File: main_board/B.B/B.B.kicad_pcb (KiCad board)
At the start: 4 copper layers, 196 x 98 mm, 249 parts, among them J2 Conn_01x10, J3 Conn_01x10, J5 USB_C_Receptacle_USB2.0, M1 Motor_DC, Q1 2N7002, Q10 2N7002, Q11 SI3447CDV, Q12 2N7002, Q2 2N7002, Q3 AO3400A, Q4 SI3447CDV, Q5 SI3447CDV, Q6 2N7002, Q7 SI3447CDV, Q8 2N7002, Q9 SI3447CDV, SW1 SW_DIP_x01, SW2 SW_DIP_x01, SW3 SW_DIP_x01, SW4 SW_DIP_x02, U1 WS2812, U10 WS2812, U11 WS2812, U12 WS2812, U13 WS2812, U14 WS2812, U15 WS2812, U16 WS2812, U17 WS2812, U18 WS2812, U19 WS2812, U2 WS2812, U20 WS2812, U21 WS2812, U22 WS2812, U23 WS2812, U24 WS2812, U25 WS2812, U26 WS2812, U27 WS2812, U28 WS2812, U29 WS2812, U3 WS2812, U30 WS2812, U31 WS2812, U32 WS2812, U33 WS2812, U34 WS2812, U35 WS2812, U36 WS2812, U37 WS2812, U38 WS2812, U39 WS2812, U4 WS2812, U40 WS2812, U41 WS2812, U42 WS2812, U43 WS2812, U44 WS2812, U45 WS2812, U46 WS2812, U47 WS2812, U48 WS2812, U49 WS2812, U5 WS2812, U50 WS2812, U51 WS2812, U52 WS2812, U53 WS2812, U54 WS2812, U55 WS2812, U56 WS2812, U57 WS2812, U58 WS2812, U59 WS2812, U6 WS2812, U60 WS2812, U61 BMX055, U62 AOZ1280, U63 FP6276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

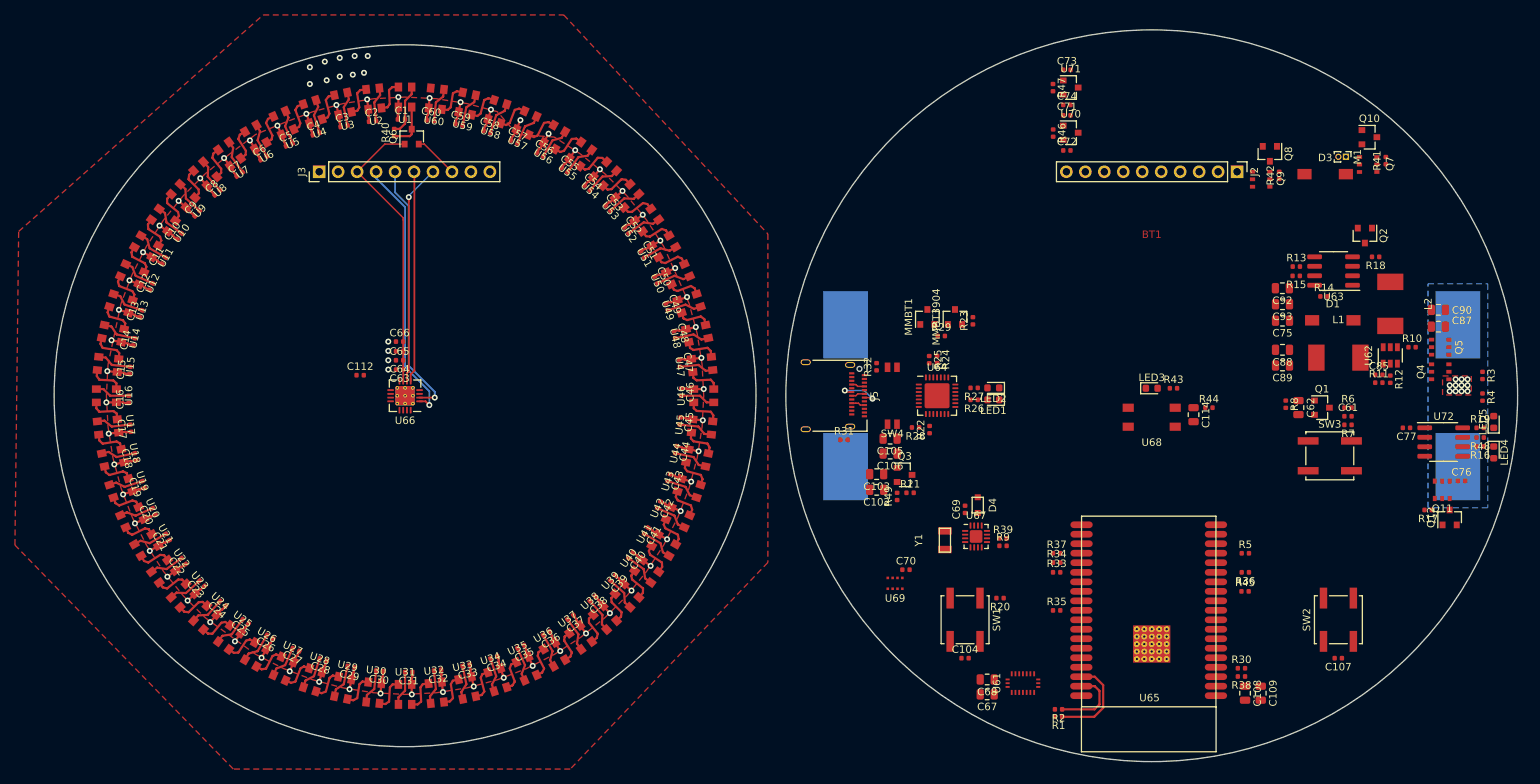
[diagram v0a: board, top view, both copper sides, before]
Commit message: PCB-0,1
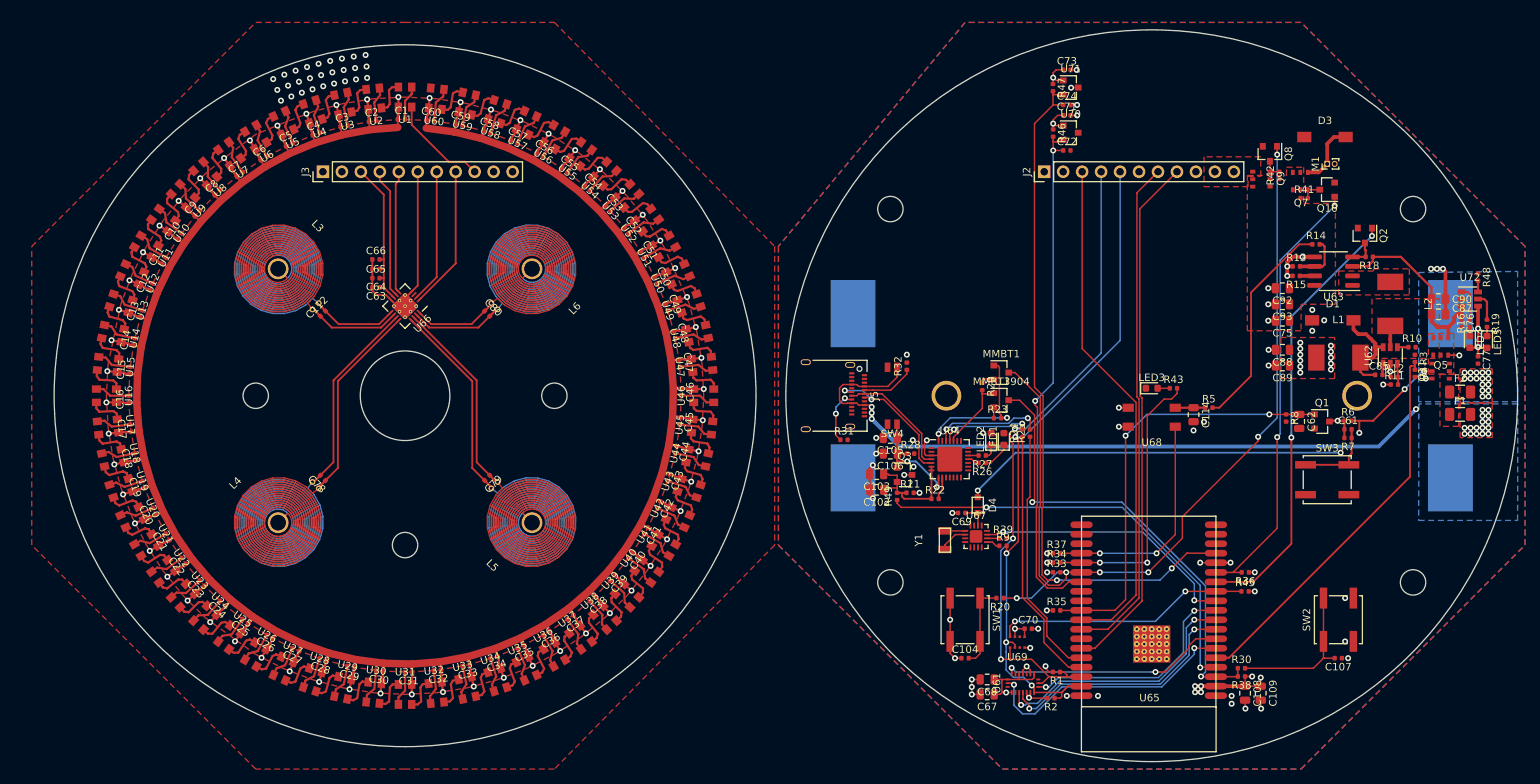
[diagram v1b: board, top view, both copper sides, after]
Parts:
- removed Q12, Q6: 2N7002, Package_TO_SOT_SMD:SOT-23
- removed Q4: SI3447CDV, BB:TSOP-6_1.5x3.0x0.95P
- removed R17: 1M, Resistor_SMD:R_0402_1005Metric
- removed R40: 7.5k, Resistor_SMD:R_0402_1005Metric
- removed R44: 220, Resistor_SMD:R_0402_1005Metric
- added C78: 1000pf, Capacitor_SMD:C_0402_1005Metric, F.Cu at (89.0, 111.0)
- added C79: 1000pf, Capacitor_SMD:C_0402_1005Metric, F.Cu at (111.0, 111.0)
- added C80: 1000pf, Capacitor_SMD:C_0402_1005Metric, F.Cu at (111.0, 89.0)
- added F1: Polyfuse, Inductor_SMD:L_1206_3216Metric, F.Cu at (241.3, 102.5)
- added F2: Polyfuse, Inductor_SMD:L_1206_3216Metric, F.Cu at (241.3, 99.5)
- added L3: L, BB:coil, F.Cu at (83.0, 83.0)
- added L4: L, BB:coil, F.Cu at (83.0, 117.0)
- added L5: L, BB:coil, F.Cu at (117.0, 117.0)
- added L6: L, BB:coil, F.Cu at (117.0, 83.0)
- C112: value C -> 1000pf
- J2, J3: value Conn_01x10 -> Conn_01x11; footprint Connector_PinHeader_2.54mm:PinHeader_1x10_P2.54mm_Vertical -> Connector_PinHeader_2.54mm:PinHeader_1x11_P2.54mm_Vertical
- R16, R19: value 1,2k -> 1k
- R31, R32: value 5k1 -> 5.1k
- R48: value 1,2k -> 2k
- R5: value 100k -> 1k
- U72: footprint Package_SO:SOP-8_3.76x4.96mm_P1.27mm -> Package_TO_SOT_SMD:SOT-23-6
- moved R48 21.5 mm to (243.7, 84.1), turned to 270 degrees
- moved C76 21.1 mm to (241.5, 90.3), turned to 270 degrees
- moved R5 20.1 mm to (207.7, 101.6)
- moved U72 19.5 mm to (242.6, 87.0)
- moved C70 18.2 mm to (183.5, 131.2)
- moved U69 18.2 mm to (182.0, 133.0)
- moved R25 16.7 mm to (183.7, 105.0), turned to 90 degrees
- moved R16 16.6 mm to (242.6, 90.3), turned to 90 degrees
- moved Q11 15.9 mm to (238.7, 96.7), turned to 270 degrees
- moved LED4 15.1 mm to (242.6, 92.8)
- moved R24 15.1 mm to (182.7, 105.0), turned to 90 degrees
- moved J2 14.4 mm to (185.6, 70.0), turned to 90 degrees
- moved R19 14.0 mm to (244.9, 90.3), turned to 270 degrees
- moved R23 13.4 mm to (179.3, 103.0), turned to 0 degrees
- moved C77 13.2 mm to (243.7, 95.2), turned to 270 degrees
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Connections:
- BT1 pad 3: Net-(BT1-Pad1) -> Net-(BT1-Pad3)
- C1 pad 1: GND -> /next-board00/GND
- C10 pad 1: GND -> /next-board00/GND
- C106 pad 1: Net-(C106-Pad1) -> Net-(C105-Pad1)
- C11 pad 1: GND -> /next-board00/GND
- C12 pad 1: GND -> /next-board00/GND
- C13 pad 1: GND -> /next-board00/GND
- C14 pad 1: GND -> /next-board00/GND
- C15 pad 1: GND -> /next-board00/GND
- C16 pad 1: GND -> /next-board00/GND
- C17 pad 1: GND -> /next-board00/GND
- C18 pad 1: GND -> /next-board00/GND
- C19 pad 1: GND -> /next-board00/GND
- C2 pad 1: GND -> /next-board00/GND
- C20 pad 1: GND -> /next-board00/GND
- C21 pad 1: GND -> /next-board00/GND
- C22 pad 1: GND -> /next-board00/GND
- C23 pad 1: GND -> /next-board00/GND
- C24 pad 1: GND -> /next-board00/GND
- C25 pad 1: GND -> /next-board00/GND
- C26 pad 1: GND -> /next-board00/GND
- C27 pad 1: GND -> /next-board00/GND
- C28 pad 1: GND -> /next-board00/GND
- C29 pad 1: GND -> /next-board00/GND
- C3 pad 1: GND -> /next-board00/GND
- C30 pad 1: GND -> /next-board00/GND
- C31 pad 1: GND -> /next-board00/GND
- C32 pad 1: GND -> /next-board00/GND
- C33 pad 1: GND -> /next-board00/GND
- C34 pad 1: GND -> /next-board00/GND
- C35 pad 1: GND -> /next-board00/GND
- C36 pad 1: GND -> /next-board00/GND
- C37 pad 1: GND -> /next-board00/GND
- C38 pad 1: GND -> /next-board00/GND
- C39 pad 1: GND -> /next-board00/GND
- C4 pad 1: GND -> /next-board00/GND
- C40 pad 1: GND -> /next-board00/GND
- C41 pad 1: GND -> /next-board00/GND
- C42 pad 1: GND -> /next-board00/GND
- C43 pad 1: GND -> /next-board00/GND
- C44 pad 1: GND -> /next-board00/GND
- C45 pad 1: GND -> /next-board00/GND
- C46 pad 1: GND -> /next-board00/GND
- C47 pad 1: GND -> /next-board00/GND
- C48 pad 1: GND -> /next-board00/GND
- C49 pad 1: GND -> /next-board00/GND
- C5 pad 1: GND -> /next-board00/GND
- C50 pad 1: GND -> /next-board00/GND
- C51 pad 1: GND -> /next-board00/GND
- C52 pad 1: GND -> /next-board00/GND
- C53 pad 1: GND -> /next-board00/GND
- C54 pad 1: GND -> /next-board00/GND
- C55 pad 1: GND -> /next-board00/GND
- C56 pad 1: GND -> /next-board00/GND
- C57 pad 1: GND -> /next-board00/GND
- C58 pad 1: GND -> /next-board00/GND
- C59 pad 1: GND -> /next-board00/GND
- C6 pad 1: GND -> /next-board00/GND
- C60 pad 1: GND -> /next-board00/GND
- C63 pad 2: GND -> /next-board00/LDC-GND
- C64 pad 2: GND -> /next-board00/LDC-GND
- C65 pad 2: GND -> /next-board00/LDC-GND
- C66 pad 1: GND -> /next-board00/LDC-GND
- C7 pad 1: GND -> /next-board00/GND
- C76 pad 1: Net-(C76-Pad1) -> /charger00/BAT
- C8 pad 1: GND -> /next-board00/GND
- C87 pad 1: Net-(C87-Pad1) -> /charger00/BAT
- C9 pad 1: GND -> /next-board00/GND
- C90 pad 1: Net-(C87-Pad1) -> /charger00/BAT
- J2 pad 1: /expanz00/5V-WS2812 -> GND
- J2 pad 10: GND -> /expanz00/5V-WS2812
- J2 pad 2: /expanz00/5V-WS2812 -> GND
- J2 pad 3: +3V3 -> /ESP3200/IO18
- J2 pad 6: /ESP3200/IO21 -> GND
- J2 pad 8: /ESP3200/IO18 -> /ESP3200/IO21
- J2 pad 9: GND -> +3V3
- J3 pad 10: GND -> /next-board00/GND
- J3 pad 4: /next-board00/SCL -> /next-board00/SHUTDOWN
- J3 pad 5: /next-board00/SDA -> /next-board00/INT
- J3 pad 6: /next-board00/INT -> /next-board00/LDC-GND
- J3 pad 7: /next-board00/SHUTDOWN -> /next-board00/SDA
- J3 pad 8: /next-board00/WS2812 -> /next-board00/SCL
- J3 pad 9: GND -> /next-board00/WS2812
- J5 pad S1: GND -> Net-(J5-PadS1)
- L2 pad 1: Net-(C87-Pad1) -> /charger00/BAT
- LED1 pad 1: GND -> Net-(LED1-Pad1)
- LED1 pad 2: Net-(LED1-Pad2) -> GND
- LED2 pad 1: GND -> Net-(LED2-Pad1)
- LED2 pad 2: Net-(LED2-Pad2) -> GND
- MMBT1 pad 3: /expanz00/ENC_OUT_1 -> /ESP3200/IO0-up
- Q11 pad 3: Net-(Q11-Pad3) -> GND
- Q11 pad 4: Net-(C76-Pad1) -> Net-(F1-Pad1)
- Q3 pad 1: Net-(C106-Pad1) -> Net-(C105-Pad1)
- Q5 pad 4: Net-(C87-Pad1) -> /charger00/BAT
- Q7 pad 1: VCC -> +5V
- Q7 pad 2: VCC -> +5V
- Q7 pad 5: VCC -> +5V
- Q7 pad 6: VCC -> +5V
- Q8 pad 1: /ESP3200/IO13 -> /ESP3200/IO0-up
- R10 pad 2: Net-(C87-Pad1) -> /charger00/BAT
- R18 pad 1: Net-(C87-Pad1) -> /charger00/BAT
- R20 pad 1: /expanz00/ENC_OUT_1 -> /ESP3200/IO0-up
- R26 pad 1: Net-(LED1-Pad2) -> Net-(LED1-Pad1)
- R27 pad 1: Net-(LED2-Pad2) -> Net-(LED2-Pad1)
- R28 pad 1: Net-(C106-Pad1) -> Net-(C105-Pad1)
- R3 pad 1: VCC -> /charger00/BAT
- R33 pad 2: /expanz00/ENC_OUT_1 -> /ESP3200/IO0-up
- R41 pad 1: VCC -> +5V
- R5 pad 1: /ESP3200/IO13 -> Net-(C114-Pad1)
- R5 pad 2: GND -> +5V
- SW4 pad 3: Net-(C106-Pad1) -> Net-(C105-Pad1)
- U1 pad 3: GND -> /next-board00/GND
- U1 pad 4: /next-board00/WS281200/DIN -> /next-board00/WS2812
- U10 pad 3: GND -> /next-board00/GND
- U11 pad 3: GND -> /next-board00/GND
- U12 pad 3: GND -> /next-board00/GND
- U13 pad 3: GND -> /next-board00/GND
- U14 pad 3: GND -> /next-board00/GND
- U15 pad 3: GND -> /next-board00/GND
- U16 pad 3: GND -> /next-board00/GND
- U17 pad 3: GND -> /next-board00/GND
- U18 pad 3: GND -> /next-board00/GND
- U19 pad 3: GND -> /next-board00/GND
- U2 pad 3: GND -> /next-board00/GND
- U20 pad 3: GND -> /next-board00/GND
- U21 pad 3: GND -> /next-board00/GND
- U22 pad 3: GND -> /next-board00/GND
- U23 pad 3: GND -> /next-board00/GND
- U24 pad 3: GND -> /next-board00/GND
- U25 pad 3: GND -> /next-board00/GND
- U26 pad 3: GND -> /next-board00/GND
- U27 pad 3: GND -> /next-board00/GND
- U28 pad 3: GND -> /next-board00/GND
- U29 pad 3: GND -> /next-board00/GND
- U3 pad 3: GND -> /next-board00/GND
- U30 pad 3: GND -> /next-board00/GND
- U31 pad 3: GND -> /next-board00/GND
- U32 pad 3: GND -> /next-board00/GND
- U33 pad 3: GND -> /next-board00/GND
- U34 pad 3: GND -> /next-board00/GND
- U35 pad 3: GND -> /next-board00/GND
- U36 pad 3: GND -> /next-board00/GND
- U37 pad 3: GND -> /next-board00/GND
- U38 pad 3: GND -> /next-board00/GND
- U39 pad 3: GND -> /next-board00/GND
- U4 pad 3: GND -> /next-board00/GND
- U40 pad 3: GND -> /next-board00/GND
- U41 pad 3: GND -> /next-board00/GND
- U42 pad 3: GND -> /next-board00/GND
- U43 pad 3: GND -> /next-board00/GND
- U44 pad 3: GND -> /next-board00/GND
- U45 pad 3: GND -> /next-board00/GND
- U46 pad 3: GND -> /next-board00/GND
- U47 pad 3: GND -> /next-board00/GND
- U48 pad 3: GND -> /next-board00/GND
- U49 pad 3: GND -> /next-board00/GND
- U5 pad 3: GND -> /next-board00/GND
- U50 pad 3: GND -> /next-board00/GND
- U51 pad 3: GND -> /next-board00/GND
- U52 pad 3: GND -> /next-board00/GND
- U53 pad 3: GND -> /next-board00/GND
- U54 pad 3: GND -> /next-board00/GND
- U55 pad 3: GND -> /next-board00/GND
- U56 pad 3: GND -> /next-board00/GND
- U57 pad 3: GND -> /next-board00/GND
- U58 pad 3: GND -> /next-board00/GND
- U59 pad 3: GND -> /next-board00/GND
- U6 pad 3: GND -> /next-board00/GND
- U60 pad 3: GND -> /next-board00/GND
- U62 pad 5: Net-(C87-Pad1) -> /charger00/BAT
- U63 pad 3: Net-(C87-Pad1) -> /charger00/BAT
- U64 pad 8: Net-(C106-Pad1) -> Net-(C105-Pad1)
- U65 pad 16: /ESP3200/IO13 -> /expanz00/ENC_OUT_1
- U65 pad 25: /expanz00/ENC_OUT_1 -> /ESP3200/IO0-up
- U66 pad 17: GND -> /next-board00/LDC-GND
- U66 pad 4: GND -> /next-board00/LDC-GND
- U66 pad 8: GND -> /next-board00/LDC-GND
- U7 pad 3: GND -> /next-board00/GND
- U72 pad 1: /ESP3200/5V_USB -> Net-(R16-Pad2)
- U72 pad 2: (no net) -> GND
- U72 pad 3: GND -> /charger00/BAT
- U72 pad 4: Net-(C76-Pad1) -> /ESP3200/5V_USB
- U72 pad 5: (no net) -> Net-(R19-Pad1)
- U72 pad 6: Net-(R16-Pad2) -> Net-(R48-Pad2)
- U8 pad 3: GND -> /next-board00/GND
- U9 pad 3: GND -> /next-board00/GND
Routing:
- net /next-board00/GND: track 0.00 -> 461.0 mm, vias 0 -> 60
- net /ESP3200/IO0-up: track 0.00 -> 120.7 mm, vias 0 -> 6
- net /ESP3200/5V_USB: track 3.61 -> 120.9 mm, vias 0 -> 6
- net GND: track 180.8 -> 68.7 mm, vias 64 -> 57
- net /expanz00/ENC_OUT_1: track 0.00 -> 94.2 mm, vias 0 -> 2
- net /ESP3200/IO23: track 9.77 -> 91.6 mm, vias 0 -> 4
- net /ESP3200/IO22: track 12.4 -> 89.3 mm, vias 0 -> 3
- net VCC: track 0.00 -> 70.5 mm, vias 0 -> 5
- net /ESP3200/IO21: track 0.00 -> 70.4 mm
- net /expanz00/ENC_OUT_0: track 0.00 -> 70.2 mm, vias 0 -> 2
- net /ESP3200/IO18: track 0.00 -> 68.4 mm
- net /ESP3200/IO19: track 0.00 -> 67.8 mm
- net /ESP3200/EN: track 0.00 -> 62.5 mm, vias 0 -> 2
- net /ESP3200/IO12-down: track 0.00 -> 59.4 mm, vias 0 -> 2
- net /ESP3200/IO14: track 0.00 -> 59.0 mm, vias 0 -> 2
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- added copper zone on F.Cu, net +3V3
- added copper zone on In2.Cu, net +3V3
- added copper zone on F.Cu, net +5V
- added copper zone on F.Cu, net /charger00/BAT
- added copper zone on F.Cu, net /expanz00/5V-WS2812
- added copper zone on In1.Cu, net /next-board00/5V
- added copper zone on F.Cu, net /next-board00/GND
- added copper zone on B.Cu, net GND
- added copper zone on In1.Cu, net GND
- added copper zone on F.Cu, net LX
- added copper zone on B.Cu, net Net-(BT1-Pad3)
- added copper zone on F.Cu, net Net-(BT1-Pad3)
- added copper zone on F.Cu, net Net-(F1-Pad1)
- added copper zone on F.Cu, net VCC
- removed copper zone on In1.Cu, net +5V
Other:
- outline, holes or cut-outs redrawn
- net class Default: clearance 0.2 -> 0.18
- rule trace_clearance: 0.2 -> 0.18
